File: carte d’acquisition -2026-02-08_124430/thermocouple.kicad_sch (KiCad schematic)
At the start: 6 parts, among them U6 MAX31855SASA_T, U6 MC74HC4067ADWR2G, U7 MC74HC4067ADWR2G

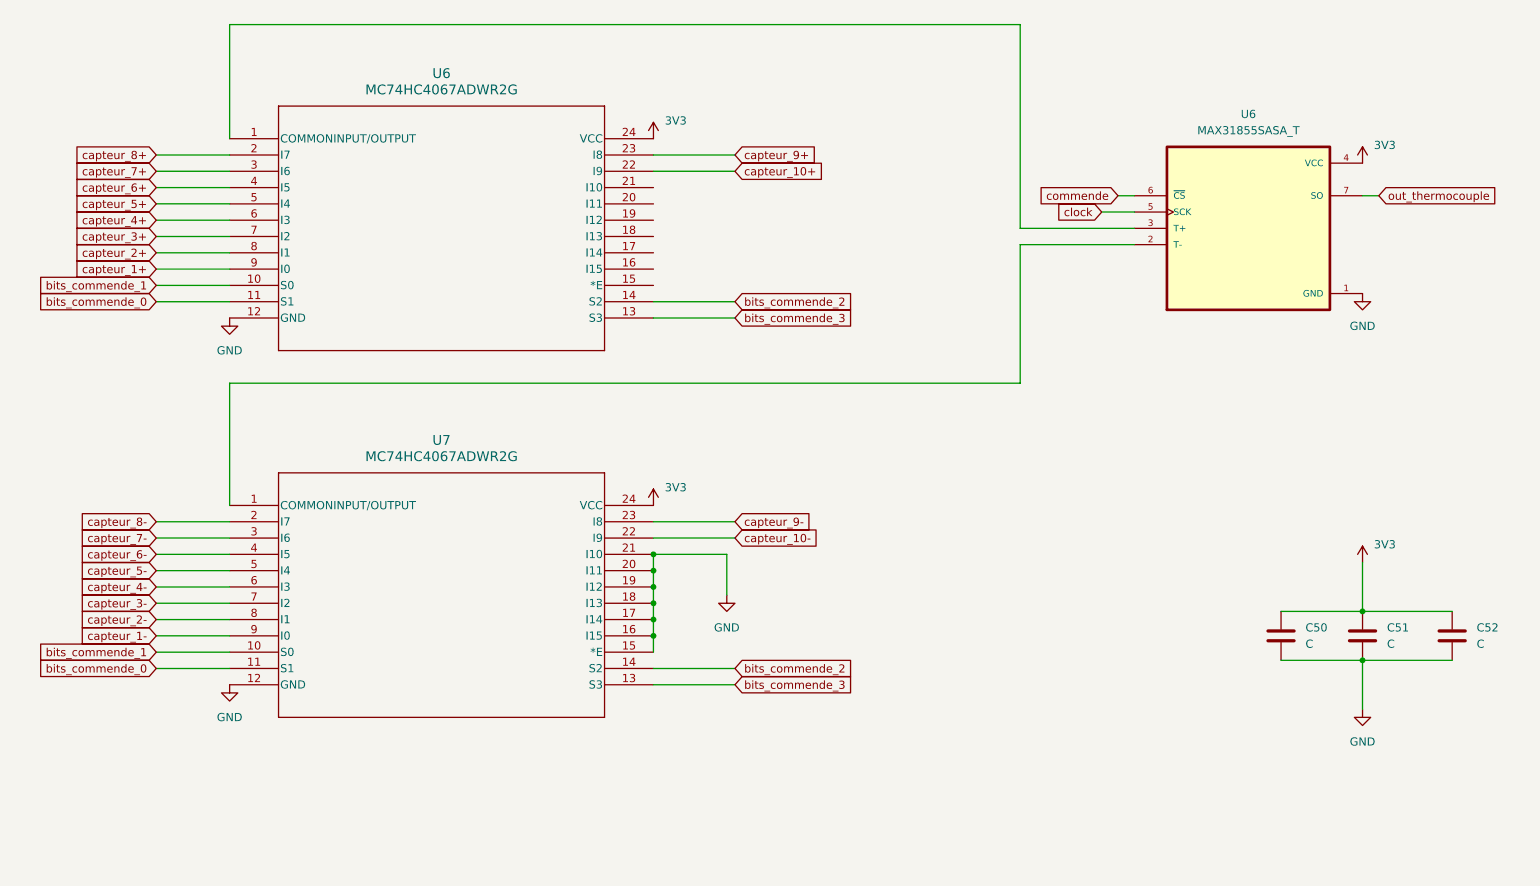
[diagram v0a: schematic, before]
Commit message: Update thermocouple.kicad_sch
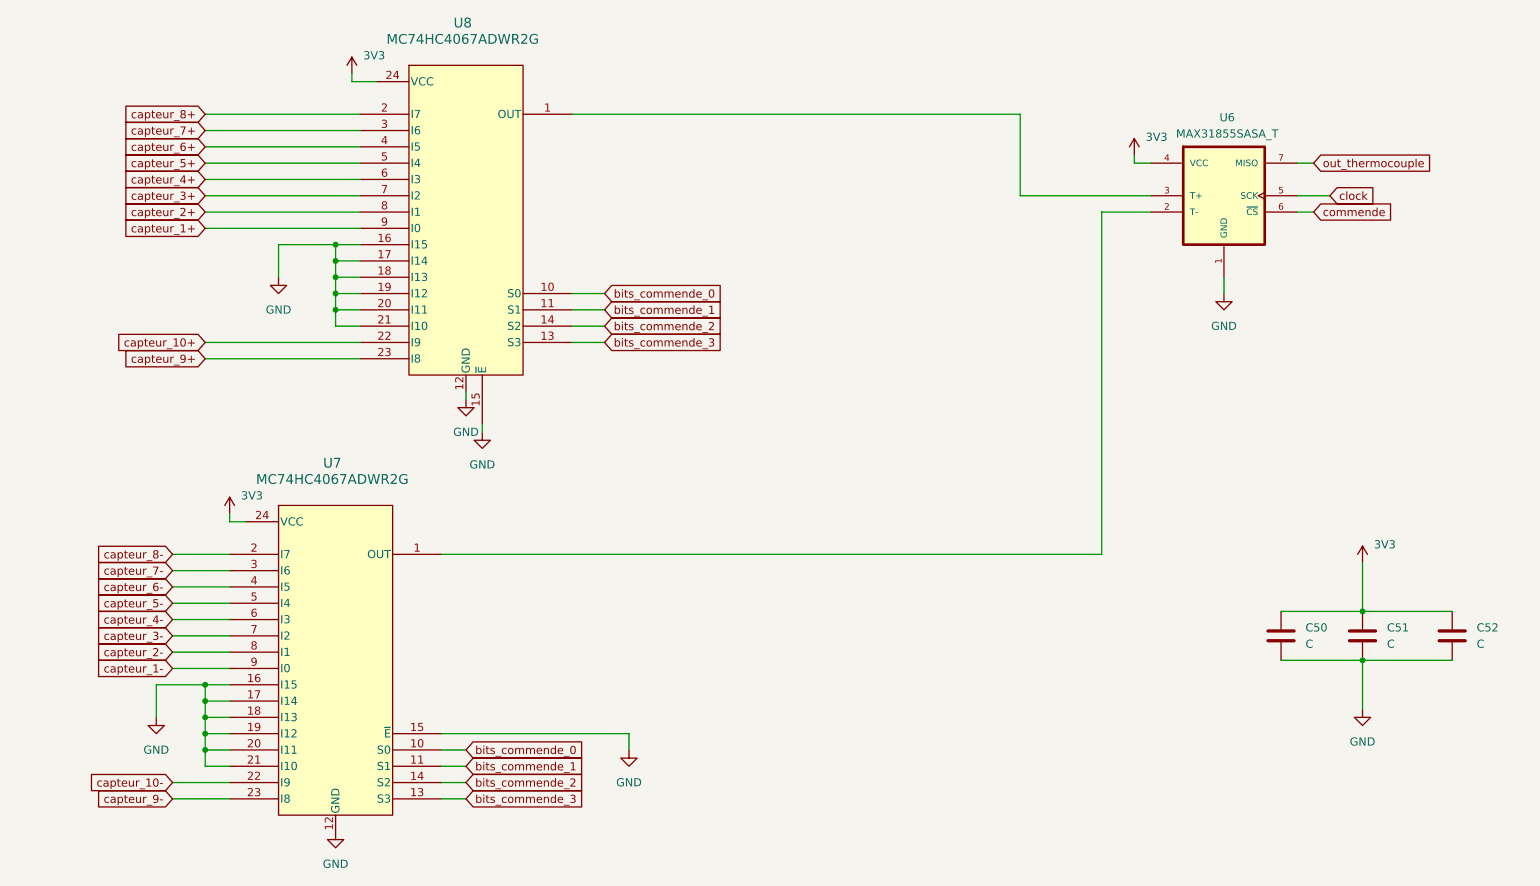
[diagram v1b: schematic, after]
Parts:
- removed U6: MC74HC4067ADWR2G, SOIC-24WB_ONS, symbol MC74HC4067ADWR2G:MC74HC4067ADWR2G
- added U8: MC74HC4067ADWR2G, footprints:SOIC-24WB_ONS, symbol MC74HC4067ADWR2G:MC74HC4067ADWR2G
- U7: footprint SOIC-24WB_ONS -> footprints:SOIC-24WB_ONS
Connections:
- net 3V3: now also U8.24 (VCC)
- net GND: now also U8.12 (GND), U8.15 (~{E}), U8.16 (I15), U8.17 (I14), U8.18 (I13), U8.19 (I12), U8.20 (I11), U8.21 (I10)
- net bits_commende_0: now also U7.10 (S0), U8.10 (S0); no longer U7.11 (S1)
- net bits_commende_1: now also U7.11 (S1), U8.11 (S1); no longer U7.10 (S0)
- net bits_commende_2: now also U8.14 (S2)
- net bits_commende_3: now also U8.13 (S3)
- net capteur_1+: now also U8.9 (I0)
- net capteur_10+: now also U8.22 (I9)
- net capteur_2+: now also U8.8 (I1)
- net capteur_3+: now also U8.7 (I2)
- net capteur_4+: now also U8.6 (I3)
- net capteur_5+: now also U8.5 (I4)
- net capteur_6+: now also U8.4 (I5)
- net capteur_7+: now also U8.3 (I6)
- net capteur_8+: now also U8.2 (I7)
- net capteur_9+: now also U8.23 (I8)
- net at U6.3 (T+): now also U8.1 (OUT)
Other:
- moved on the sheet: U6
